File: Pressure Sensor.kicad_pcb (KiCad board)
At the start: 2 copper layers, 41.9 x 24.1 mm, 5 parts, among them J1 Conn_01x03_Female, U1 MPXV7025DP

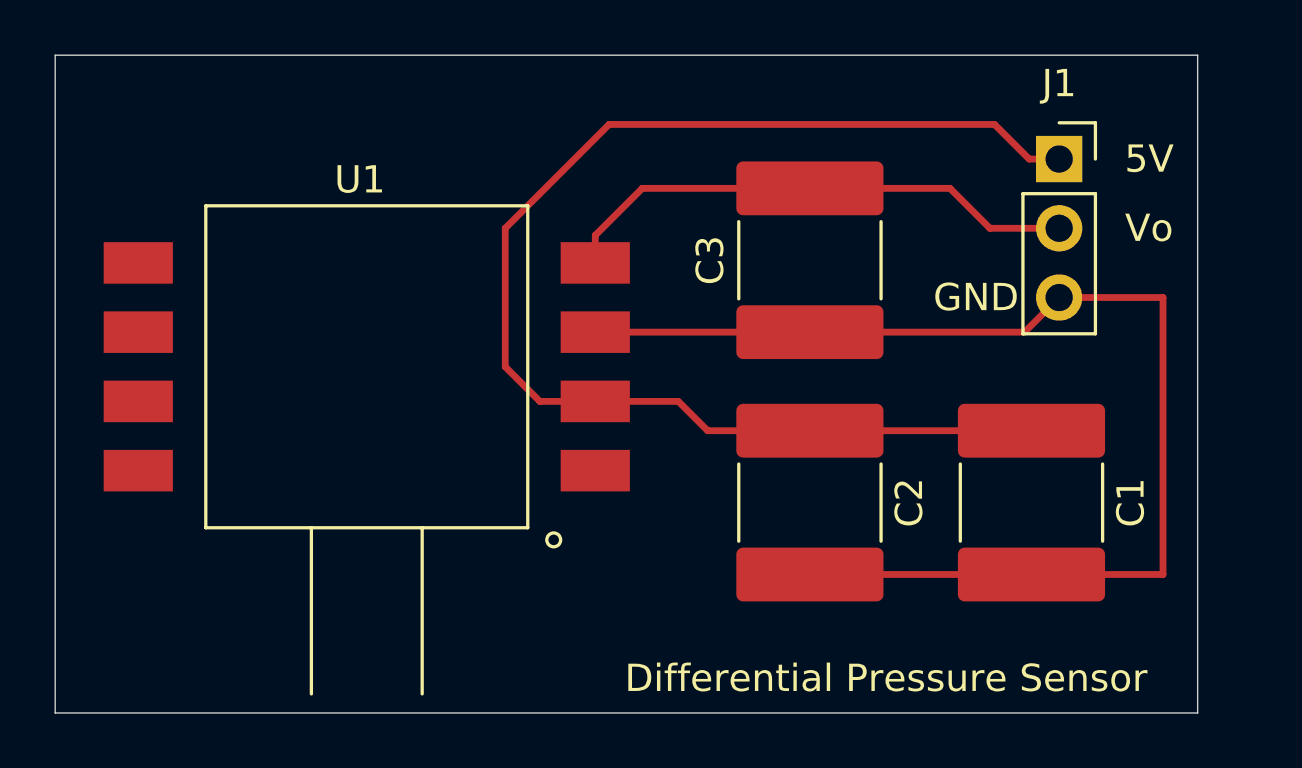
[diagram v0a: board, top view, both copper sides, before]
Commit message: updated caps
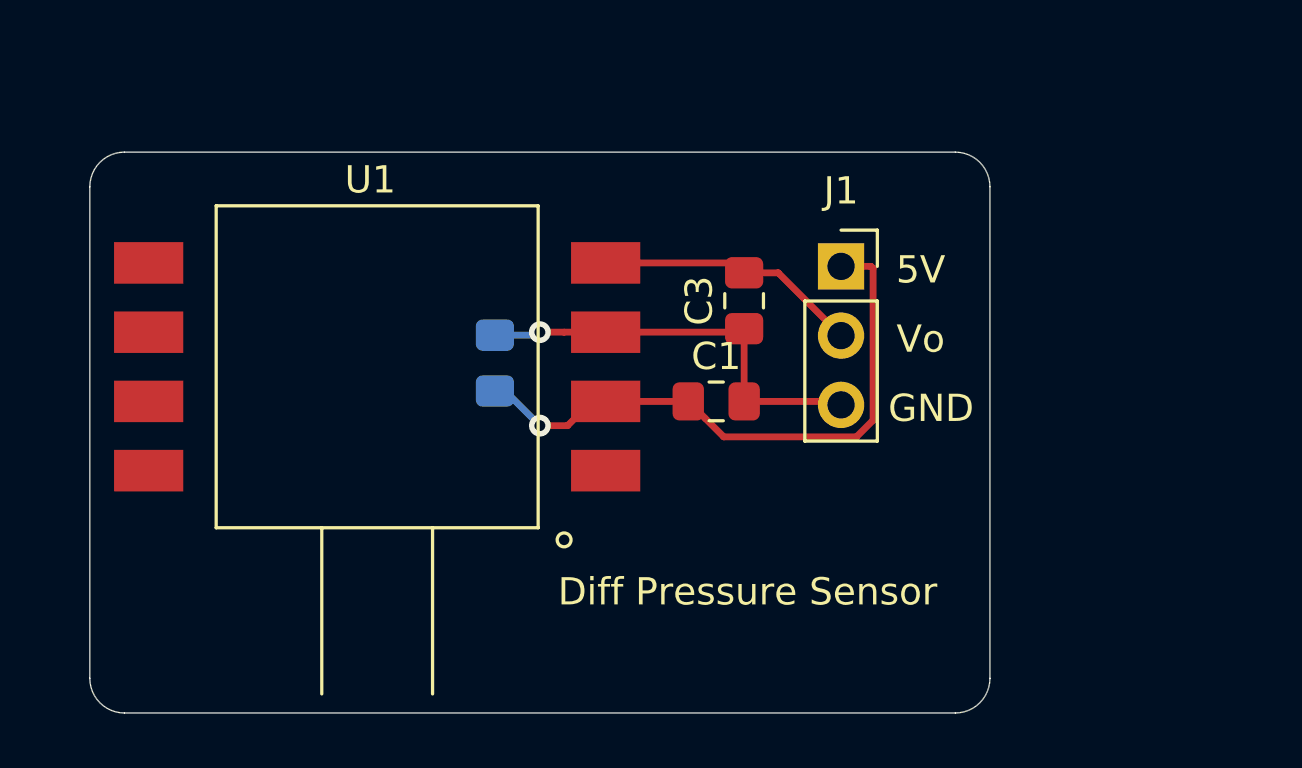
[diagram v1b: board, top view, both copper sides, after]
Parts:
- C1, C3: footprint Capacitor_SMD:C_2220_5650Metric_Pad1.97x5.40mm_HandSolder -> Capacitor_SMD:C_0805_2012Metric_Pad1.15x1.40mm_HandSolder
- C2: footprint Capacitor_SMD:C_2220_5650Metric_Pad1.97x5.40mm_HandSolder -> Capacitor_SMD:C_0805_2012Metric_Pad1.15x1.40mm_HandSolder; moved to B.Cu
- moved C2 12.6 mm to (136.8, 26.5), turned to 90 degrees
- moved C1 12.1 mm to (144.9, 27.9), turned to 0 degrees
- moved J1 8.92 mm to (149.5, 23.0)
- moved C3 2.83 mm to (145.9, 24.2)
- moved U1 0.38 mm to (132.5, 26.7)
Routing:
- net GND: track 42.9 -> 15.6 mm, vias 0 -> 1
- net +5V: track 48.8 -> 22.3 mm, vias 0 -> 1
- net output: track 19.4 -> 9.74 mm
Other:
- board size 41.9 x 24.1 mm -> 33 x 20.6 mm
- board text added: "Diff Pressure Sensor"
- board text removed: "Differential Pressure Sensor"
